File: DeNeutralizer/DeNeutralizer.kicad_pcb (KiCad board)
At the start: 2 copper layers, 27.9 x 72 mm, 21 parts, among them J1 Screw_Terminal_01x03, J2 Screw_Terminal_01x03, J3 Screw_Terminal_01x03, J4 Screw_Terminal_01x03, J5 Screw_Terminal_01x02, J6 Screw_Terminal_01x05, J7 Screw_Terminal_01x02, J8 Conn_01x02_Male, J9 Ripple-Cap, U1 PC817

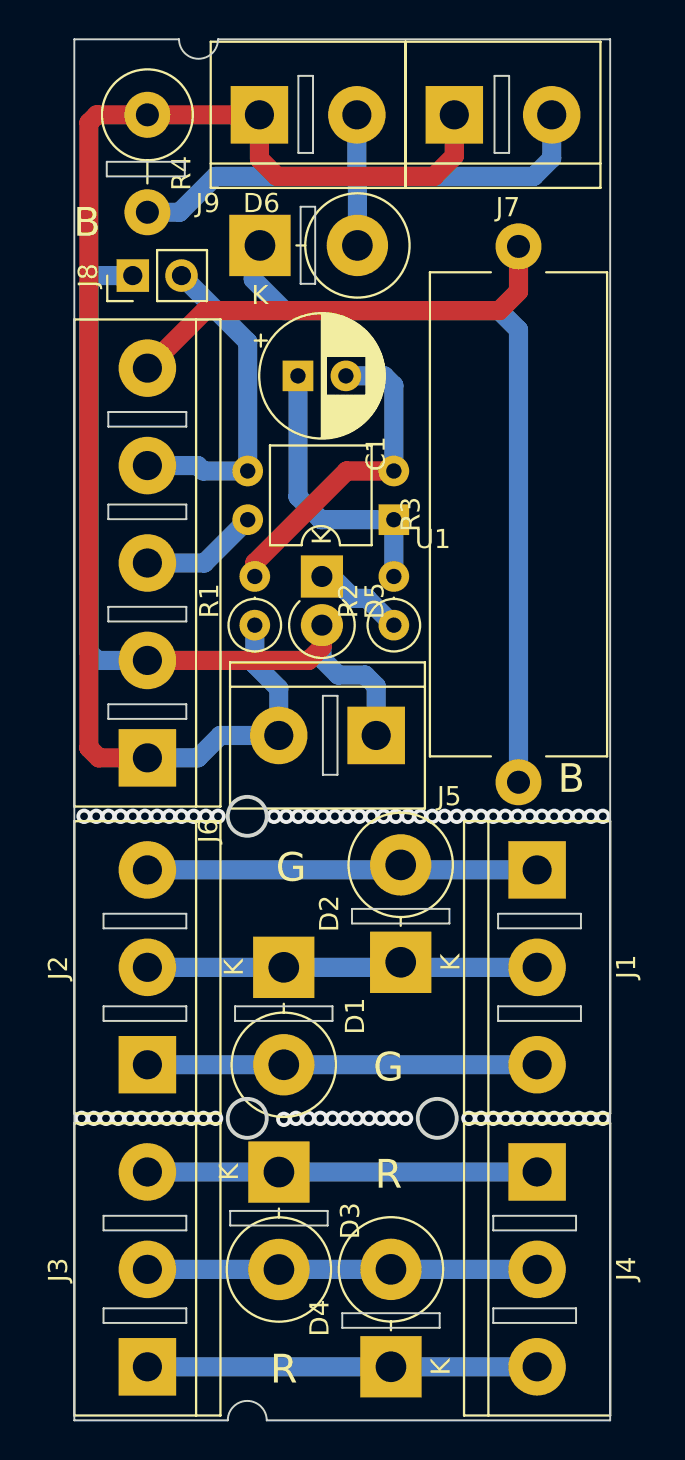
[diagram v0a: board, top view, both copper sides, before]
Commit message: Make tha board as low profile as it can for this time :D
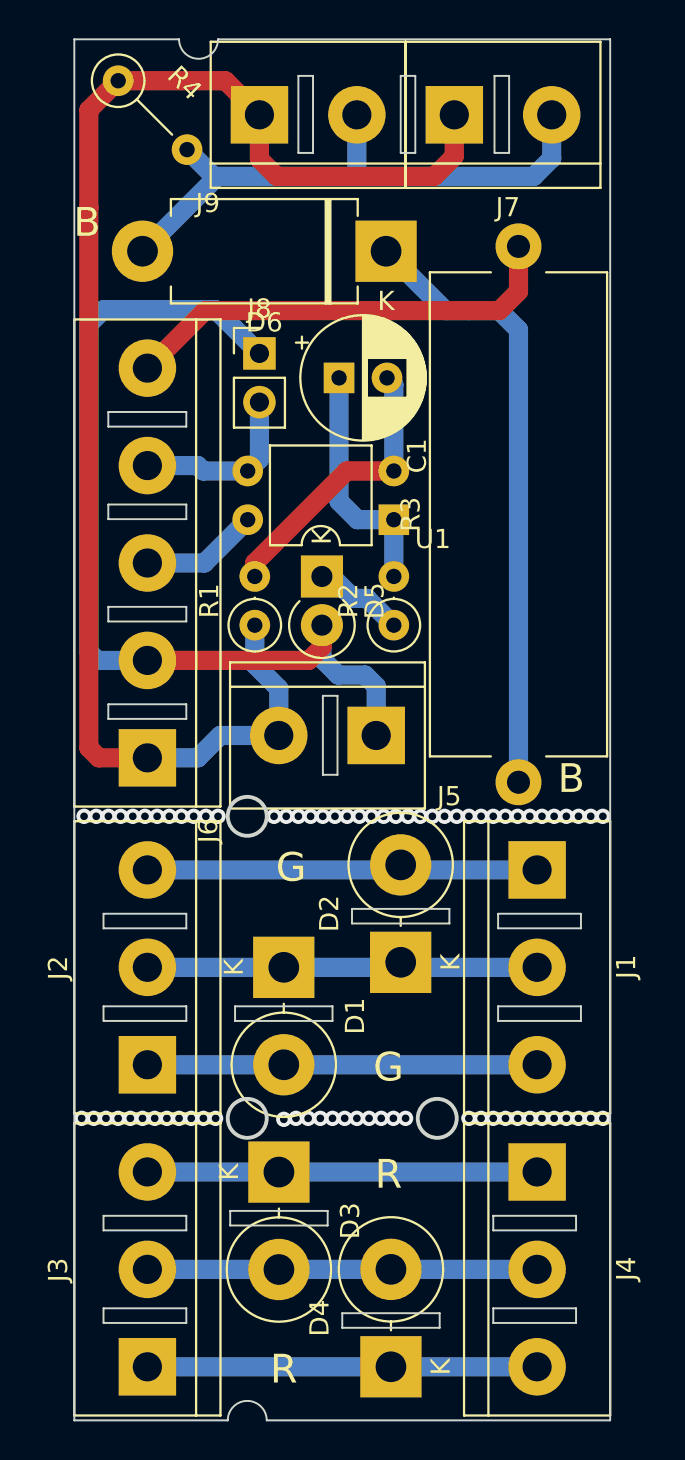
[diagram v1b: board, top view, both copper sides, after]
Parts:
- D6: footprint Diode_THT:D_DO-201AD_P5.08mm_Vertical_KathodeUp -> Diode_THT:D_DO-201AD_P12.70mm_Horizontal
- R4: footprint Resistor_THT:R_Axial_DIN0414_L11.9mm_D4.5mm_P5.08mm_Vertical -> Resistor_THT:R_Axial_DIN0207_L6.3mm_D2.5mm_P5.08mm_Vertical
- moved J8 7.75 mm to (126.5, 84.8), turned to 0 degrees
- moved D6 6.58 mm to (133.1, 79.5), turned to 180 degrees
- moved R4 2.34 mm to (119.1, 70.6), turned to -45 degrees
- moved C1 2.15 mm to (130.6, 86.1)
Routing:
- net Net-(D6-K): track 40.2 -> 32.2 mm
- net Net-(J6-Pin_4): track 17.0 -> 9.19 mm
- net Net-(D5-A): track 43.2 -> 48.8 mm
- net Net-(C1-Pad2): track 17.1 -> 14.9 mm
- net Net-(C1-Pad1): track 14.8 -> 12.7 mm
- net Net-(J5-Pin_2): track 74.0 -> 75.8 mm
- net Net-(D6-A): track 31.5 -> 31.0 mm
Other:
- outline, holes or cut-outs redrawn

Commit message: Add 3D model of the Shelly
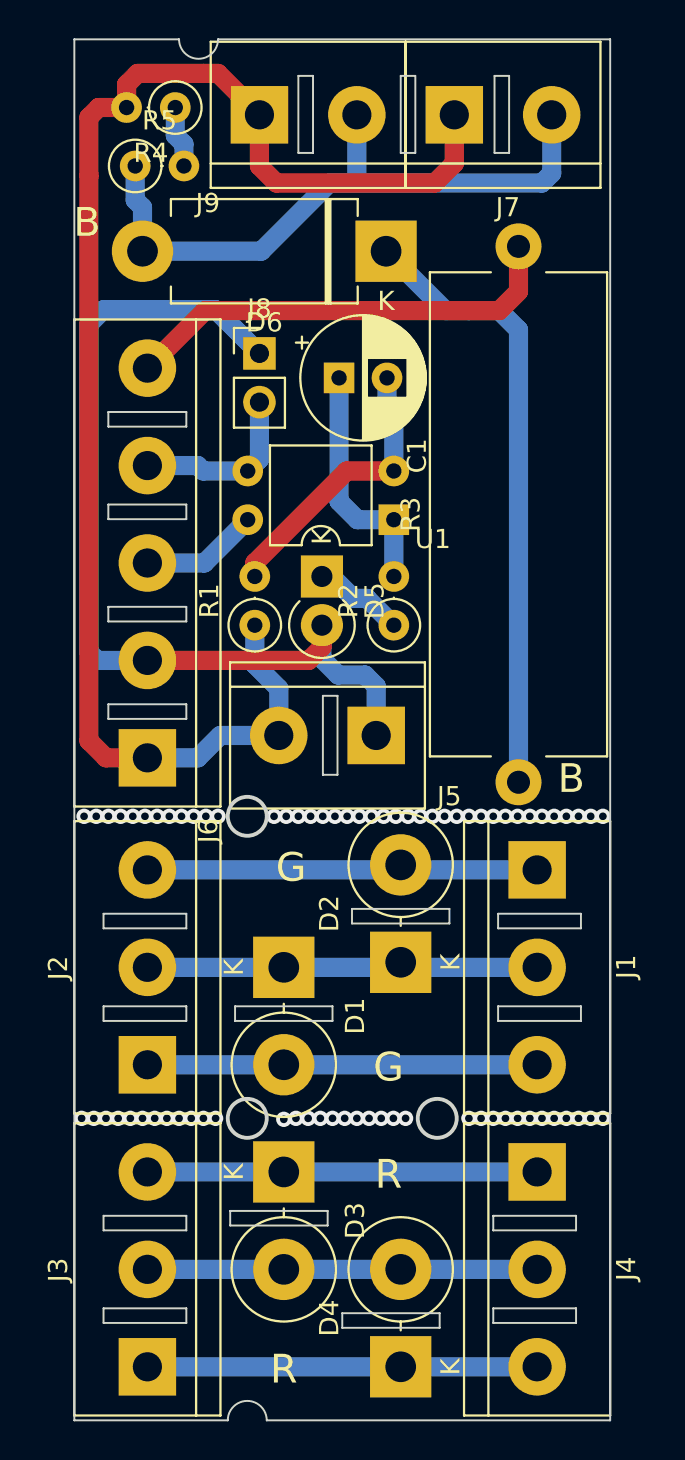
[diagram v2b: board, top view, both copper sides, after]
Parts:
- added R5: 500k, Resistor_THT:R_Axial_DIN0207_L6.3mm_D2.5mm_P2.54mm_Vertical, F.Cu at (120.0, 75.1)
- J5: value Screw_Terminal_01x02 -> Power
- J7: value Screw_Terminal_01x02 -> Load
- R3: value 10/5W -> 5/5W
- R4: value 1M/0.6W -> 500k; footprint Resistor_THT:R_Axial_DIN0207_L6.3mm_D2.5mm_P5.08mm_Vertical -> Resistor_THT:R_Axial_DIN0207_L6.3mm_D2.5mm_P2.54mm_Vertical
- moved R4 3.29 mm to (122.1, 72.0), turned to 180 degrees
- moved D4 0.51 mm to (133.9, 137.7)
- moved D3 0.25 mm to (127.8, 127.5)
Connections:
- R3 pad 1: Net-(D6-K) -> Net-(F1-Pad1)
- R4 pad 1: Net-(J5-Pin_2) -> Net-(R4-Pad1)
- R4 pad 2: Net-(D6-A) -> Net-(J5-Pin_2)
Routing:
- net Net-(R4-Pad1): track 0.00 -> 3.23 mm
- net Net-(D6-A): track 31.0 -> 34.1 mm
- net Net-(J5-Pin_2): track 75.8 -> 77.5 mm
